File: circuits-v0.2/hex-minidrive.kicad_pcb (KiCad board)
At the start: 2 copper layers, 30 x 30 mm, 14 parts

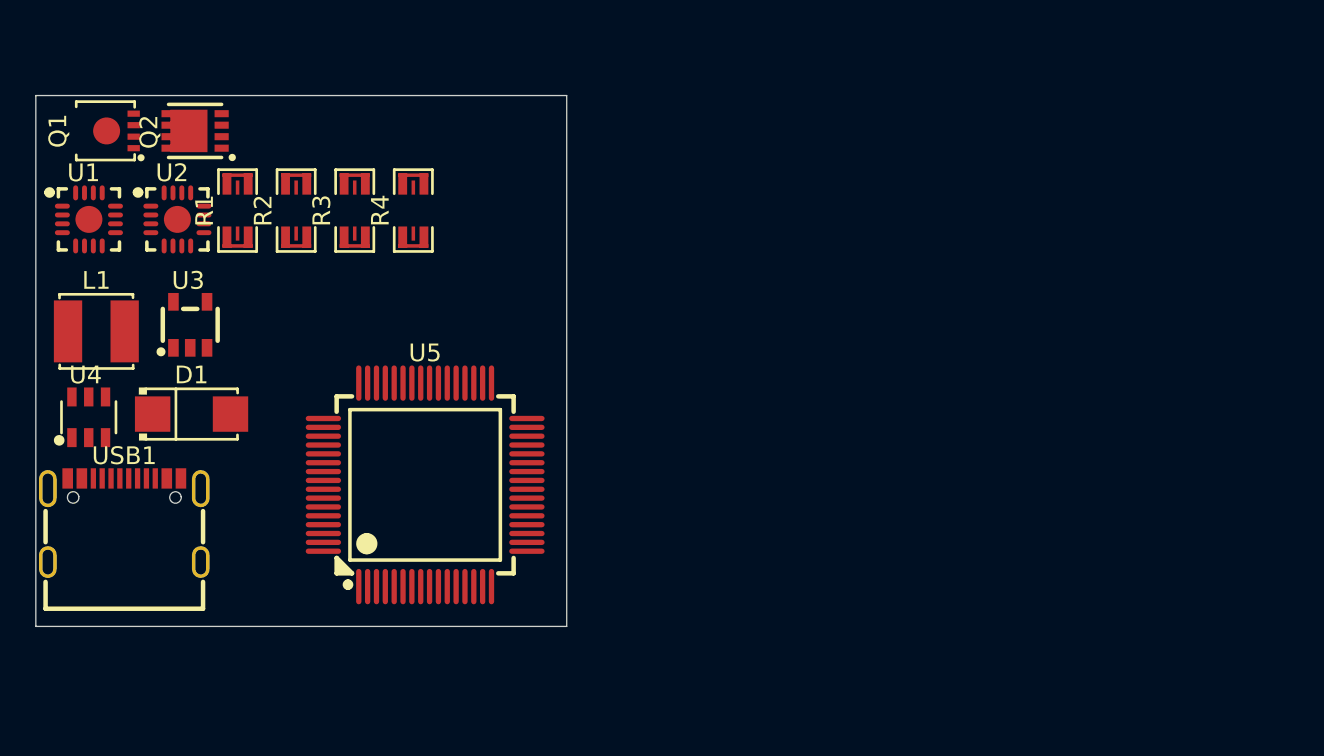
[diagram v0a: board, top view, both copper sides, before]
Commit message: Tentatively finish new schematic.
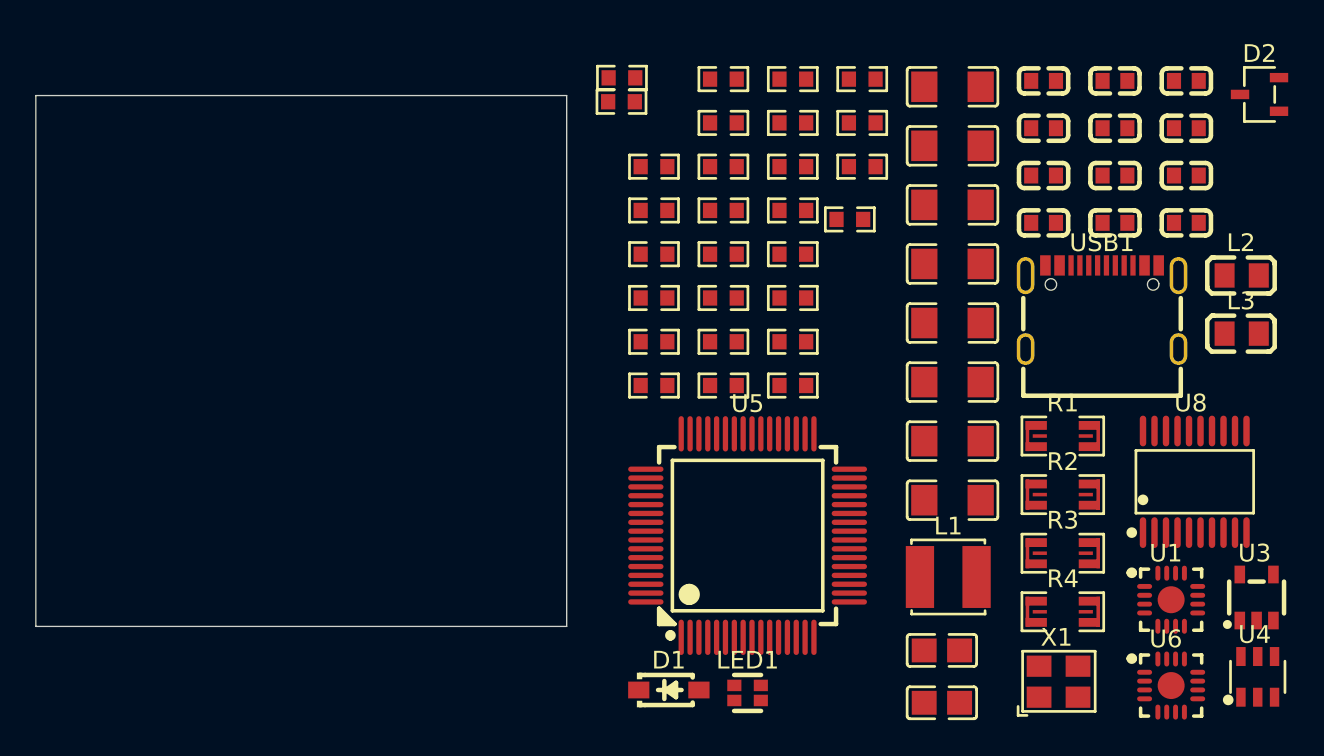
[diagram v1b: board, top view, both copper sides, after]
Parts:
- removed Q1: ~, Library:DFN-8_L3.3-W3.3-P0.65-BL-2
- removed Q2: ~, Library:DFN-8_L3.0-W3.0-P0.65-BL
- removed U2: ~, Library:QFN-16_L3.0-W3.0-P0.50-TL-EP1.7
- added C10: 10uF, Library:C1206, F.Cu at (97.8, 43.8)
- added C11: 10uF, Library:C1206, F.Cu at (97.8, 47.2)
- added C12: 1uF, Library:C0603, F.Cu at (107.0, 40.2)
- added C14: 10uF, Library:C1206, F.Cu at (97.8, 50.5)
- added C15: 10uF, Library:C1206, F.Cu at (97.8, 53.9)
- added C16: 10uF, Library:C1206, F.Cu at (97.8, 57.2)
- added C17: 10uF, Library:C1206, F.Cu at (97.8, 60.5)
- added C20: 15pF, Library:C0603, F.Cu at (107.0, 42.8)
- added C21: 15pF, Library:C0603, F.Cu at (107.0, 45.5)
- added C23: 1uF, Library:C0603, F.Cu at (107.0, 48.2)
- added C28: 10uF, Library:C1206, F.Cu at (97.8, 63.9)
- added C3: 10uF, Library:C1206, F.Cu at (97.8, 40.5)
- added C30: 1nF, Library:C0603, F.Cu at (111.0, 40.2)
- added C31: 1nF, Library:C0603, F.Cu at (111.0, 42.8)
- added C32: 1nF, Library:C0603, F.Cu at (111.0, 45.5)
- added C33: 1nF, Library:C0603, F.Cu at (111.0, 48.2)
- added C4: 22uF, Library:C0805, F.Cu at (97.2, 72.4)
- added C5: 22uF, Library:C0805, F.Cu at (97.2, 75.3)
- added C6: 100pF, Library:C0603, F.Cu at (102.9, 40.2)
- added C7: 1uF, Library:C0603, F.Cu at (102.9, 42.8)
- added C8: 1uF, Library:C0603, F.Cu at (102.9, 45.5)
- added C9: 10nF, Library:C0603, F.Cu at (102.9, 48.2)
- added D2: ~, Library:SOT-23-3_L3.0-W1.7-P0.95-LS2.9-BR, F.Cu at (115.2, 40.9)
- added L2: 10uH, Library:L0805, F.Cu at (114.1, 51.2)
- added L3: 300mΩ, Library:L0805, F.Cu at (114.1, 54.5)
- added LED1: ~, Library:LED-ARRAY-SMD_4P-L1.6-W1.5-BR_XL-1615RGBC-RF, F.Cu at (86.2, 74.8)
- added R10: 49.9Ω, Library:R0603, F.Cu at (80.9, 52.4)
- added R11: 1.5kΩ, Library:R0603, F.Cu at (80.9, 54.9)
- added R12: 1.5kΩ, Library:R0603, F.Cu at (80.9, 57.4)
- added R13: 1.5kΩ, Library:R0603, F.Cu at (84.9, 40.1)
- added R14: 10Ω, Library:R0603, F.Cu at (84.9, 42.5)
- added R15: 10Ω, Library:R0603, F.Cu at (84.9, 45.0)
- added R16: 10kΩ, Library:R0603, F.Cu at (84.9, 47.5)
- added R17: 100kΩ, Library:R0603, F.Cu at (84.9, 50.0)
- added R18: 10kΩ, Library:R0603, F.Cu at (84.9, 52.4)
- added R19: 10kΩ, Library:R0603, F.Cu at (84.9, 54.9)
- added R20: 10Ω, Library:R0603, F.Cu at (84.9, 57.4)
- added R21: 100kΩ, Library:R0603, F.Cu at (88.8, 40.1)
- added R22: 10Ω, Library:R0603, F.Cu at (88.8, 42.5)
- added R23: 10Ω, Library:R0603, F.Cu at (88.8, 45.0)
- added R24: 10Ω, Library:R0603, F.Cu at (88.8, 47.5)
- added R25: 5.1kΩ, Library:R0603, F.Cu at (88.8, 50.0)
- added R26: 10Ω, Library:R0603, F.Cu at (88.8, 52.4)
- added R27: 10Ω, Library:R0603, F.Cu at (88.8, 54.9)
- added R28: 100kΩ, Library:R0603, F.Cu at (88.8, 57.4)
- added R29: 10Ω, Library:R0603, F.Cu at (92.7, 40.1)
- added R30: 5.1kΩ, Library:R0603, F.Cu at (92.7, 42.5)
- added R31: 100kΩ, Library:R0603, F.Cu at (92.7, 45.0)
- added R33: 5.1kΩ, Library:R0603, F.Cu at (92.0, 48.0)
- added R5: 100kΩ, Library:R0603, F.Cu at (79.1, 40.0)
- added R6: 13kΩ, Library:R0603, F.Cu at (79.1, 41.4)
- added R7: 5.1kΩ, Library:R0603, F.Cu at (80.9, 45.0)
- added R8: 5.1kΩ, Library:R0603, F.Cu at (80.9, 47.5)
- added R9: 10Ω, Library:R0603, F.Cu at (80.9, 50.0)
- added U6: ~, Library:QFN-16_L3.0-W3.0-P0.50-TL-EP1.7, F.Cu at (110.2, 74.3)
- added U8: ~, Library:TSSOP-20_L6.5-W4.4-P0.65-LS6.4-BL, F.Cu at (111.5, 62.8)
- added X1: 16MHz, Library:OSC-SMD_4P-L3.2-W2.5-BL, F.Cu at (103.8, 74.1)
- D1: footprint Library:SMA_L4.3-W2.6-LS5.2-RD -> Library:SOD-123_L2.7-W1.6-LS3.7-RD-1
- moved U4 67.7 mm to (115.0, 73.9)
- moved U1 64.8 mm to (110.2, 69.5)
- moved U3 62.2 mm to (115.0, 69.4)
- moved USB1 56.5 mm to (106.3, 53.0)
- moved L1 50.1 mm to (97.6, 68.2)
- moved R1 48.3 mm to (104.0, 60.2), turned to 0 degrees
- moved R2 46.2 mm to (104.0, 63.6), turned to 0 degrees
- moved R3 44.5 mm to (104.0, 66.9), turned to 0 degrees
- moved R4 43.1 mm to (104.0, 70.2), turned to 0 degrees
- moved D1 31.2 mm to (81.8, 74.6)
- moved U5 18.4 mm to (86.2, 65.9)
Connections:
- D1 pad 1: unconnected-(D1-K-Pad1) -> 5V
- D1 pad 2: unconnected-(D1-A-Pad2) -> Net-(D1-+)
- L1 pad 1: unconnected-(L1-Pad1) -> Net-(U4-SW)
- L1 pad 2: unconnected-(L1-Pad2) -> 5V
- R1 pad 1: unconnected-(R1-Shunt-1-Pad1) -> Net-(Q1-S)
- R1 pad 2: unconnected-(R1-Shunt-2-Pad2) -> GND
- R1 pad 3: unconnected-(R1-Probe-1-Pad3) -> +Probe-1
- R1 pad 4: unconnected-(R1-Probe-2-Pad4) -> -Probe-1
- R2 pad 1: unconnected-(R2-Shunt-1-Pad1) -> Net-(Q3-S)
- R2 pad 2: unconnected-(R2-Shunt-2-Pad2) -> GND
- R2 pad 3: unconnected-(R2-Probe-1-Pad3) -> +Probe-2
- R2 pad 4: unconnected-(R2-Probe-2-Pad4) -> -Probe-2
- R3 pad 1: unconnected-(R3-Shunt-1-Pad1) -> Net-(Q5-S)
- R3 pad 2: unconnected-(R3-Shunt-2-Pad2) -> GND
- R3 pad 3: unconnected-(R3-Probe-1-Pad3) -> +Probe-3
- R3 pad 4: unconnected-(R3-Probe-2-Pad4) -> -Probe-3
- R4 pad 1: unconnected-(R4-Shunt-1-Pad1) -> Net-(Q7-S)
- R4 pad 2: unconnected-(R4-Shunt-2-Pad2) -> GND
- R4 pad 3: unconnected-(R4-Probe-1-Pad3) -> +Probe-4
- R4 pad 4: unconnected-(R4-Probe-2-Pad4) -> -Probe-4
- U1 pad 1: unconnected-(U1-HIN1-Pad1) -> TIM1_CH1
- U1 pad 10: unconnected-(U1-HO2-Pad10) -> P-Gate-2
- U1 pad 11: unconnected-(U1-LO2-Pad11) -> N-Gate-2
- U1 pad 14: unconnected-(U1-GND-Pad14) -> GND
- U1 pad 16: unconnected-(U1-HIN2-Pad16) -> TIM1_CH2
- U1 pad 3: unconnected-(U1-LIN2-Pad3) -> TIM1_CH2N
- U1 pad 4: unconnected-(U1-LIN1-Pad4) -> TIM1_CH1N
- U1 pad 6: unconnected-(U1-VCC1-Pad6) -> Net-(U1-VCC1)
- U1 pad 7: unconnected-(U1-VCC2-Pad7) -> VCC
- U1 pad 8: unconnected-(U1-HO1-Pad8) -> P-Gate-1
- U1 pad 9: unconnected-(U1-LO1-Pad9) -> N-Gate-1
- U3 pad 1: unconnected-(U3-IN-Pad1) -> 5V
- U3 pad 2: unconnected-(U3-GND-Pad2) -> GND
- U3 pad 3: unconnected-(U3-EN-Pad3) -> 5V
- U3 pad 4: unconnected-(U3-BYP-Pad4) -> Net-(U3-BYP)
- U3 pad 5: unconnected-(U3-OUT-Pad5) -> 3V3
- U4 pad 1: unconnected-(U4-GND-Pad1) -> GND
- U4 pad 2: unconnected-(U4-SW-Pad2) -> Net-(U4-SW)
- U4 pad 3: unconnected-(U4-VIN-Pad3) -> VCC
- U4 pad 4: unconnected-(U4-FB-Pad4) -> Buck-FB
- U4 pad 6: unconnected-(U4-BOOT-Pad6) -> Net-(U4-BOOT)
- U5 pad 16: unconnected-(U5-VDD-Pad16) -> 3V3
- U5 pad 32: unconnected-(U5-VDD-Pad32) -> 3V3
- U5 pad 48: unconnected-(U5-VDD-Pad48) -> 3V3
- U5 pad 5: unconnected-(U5-PF0-OSC_IN-Pad5) -> Net-(U5-PF0-OSC_IN)
- U5 pad 6: unconnected-(U5-PF1-OSC_OUT-Pad6) -> Net-(U5-PF1-OSC_OUT)
- U5 pad 64: unconnected-(U5-VDD-Pad64) -> 3V3
- USB1 pad A1B12: unconnected-(USB1-GND-PadA1B12) -> GND
- USB1 pad A4B9: unconnected-(USB1-VBUS-PadA4B9) -> USB:5V
- USB1 pad A5: unconnected-(USB1-CC1-PadA5) -> Net-(USB1-CC1)
- USB1 pad A6: unconnected-(USB1-DP1-PadA6) -> USB_D_P
- USB1 pad A7: unconnected-(USB1-DN1-PadA7) -> USB_D_N
- USB1 pad B1A12: unconnected-(USB1-GND-PadB1A12) -> GND
- USB1 pad B4A9: unconnected-(USB1-VBUS-PadB4A9) -> USB:5V
- USB1 pad B5: unconnected-(USB1-CC2-PadB5) -> Net-(USB1-CC2)
- USB1 pad B6: unconnected-(USB1-DP2-PadB6) -> USB_D_P
- USB1 pad B7: unconnected-(USB1-DN2-PadB7) -> USB_D_N

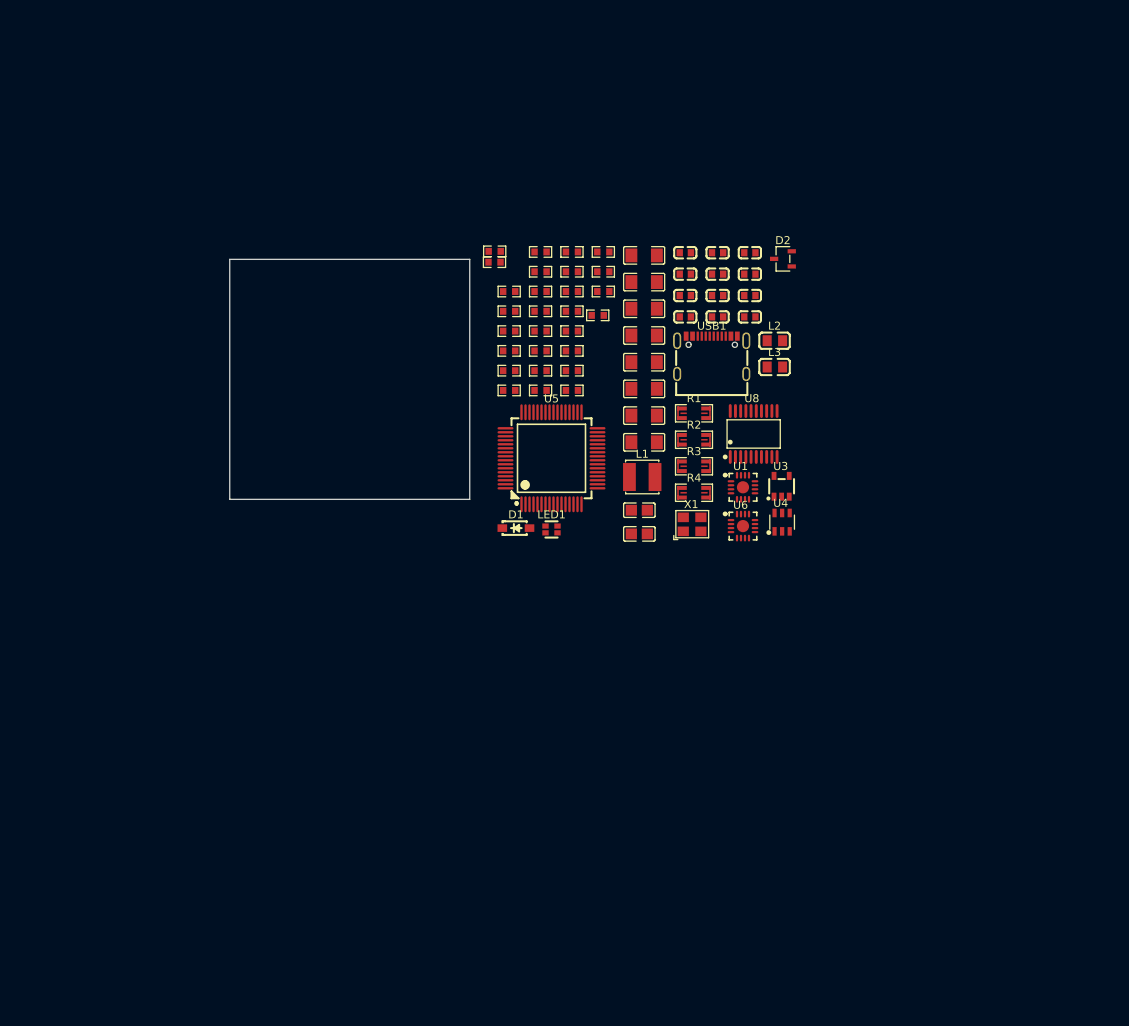
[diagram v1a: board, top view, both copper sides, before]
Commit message: Finish the new version schematic.
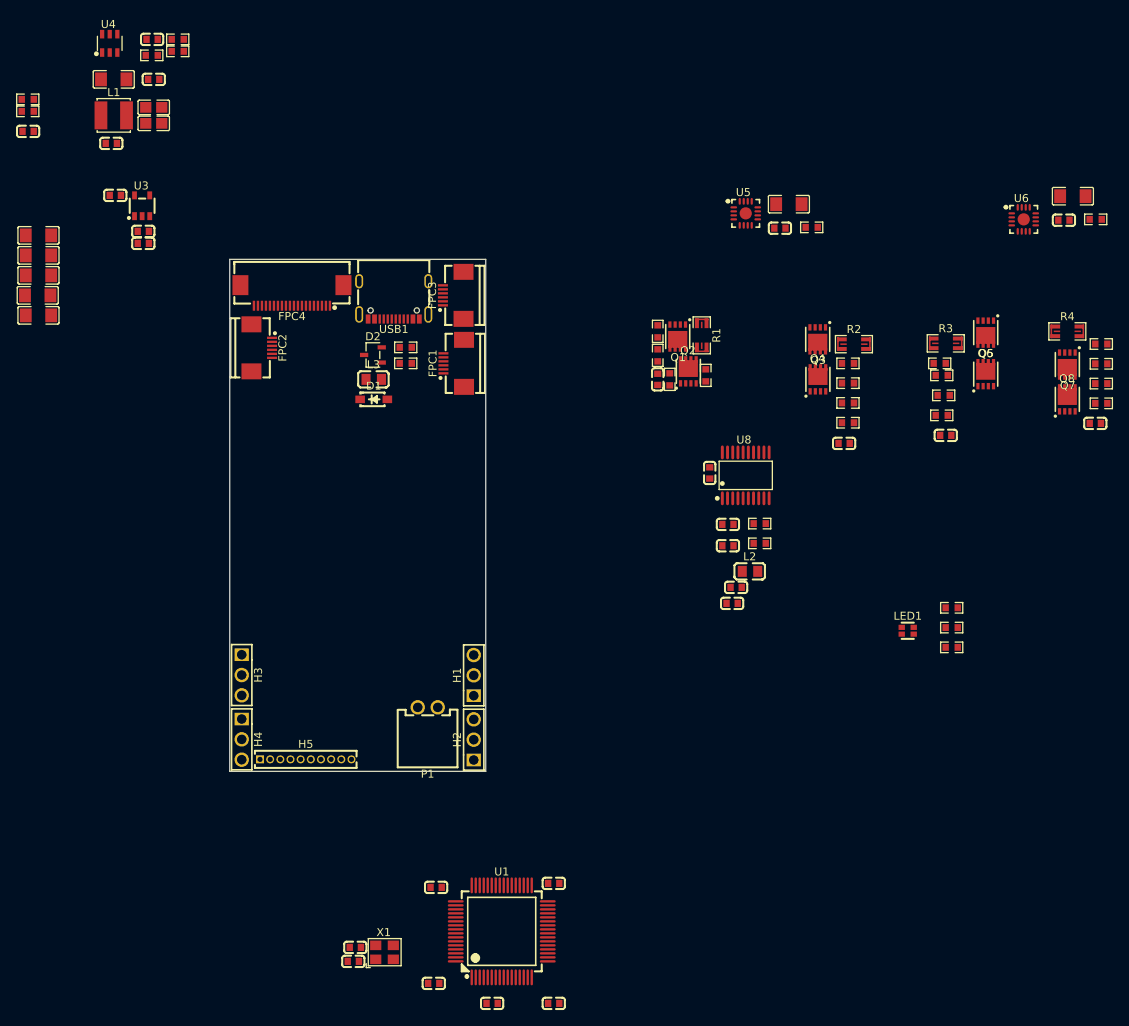
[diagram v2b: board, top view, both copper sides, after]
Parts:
- removed C17, C28: 10uF, Library:C1206
- removed C23: 1uF, Library:C0603
- removed C31, C32, C33: 1nF, Library:C0603
- removed R13: 1.5kΩ, Library:R0603
- removed R14, R15, R20, R24, R26, R27, R29, R9: 10Ω, Library:R0603
- removed R16, R19: 10kΩ, Library:R0603
- removed R25, R30, R33, R7, R8: 5.1kΩ, Library:R0603
- removed R28, R31: 100kΩ, Library:R0603
- added C1: 100nF, Library:C0603, F.Cu at (31.2, 26.5)
- added C101: 1nF, Library:C0603, F.Cu at (99.5, 56.0)
- added C13: 100nF, Library:C0603, F.Cu at (108.8, 84.0)
- added C2: 100nF, Library:C0603, F.Cu at (36.5, 18.5)
- added C201: 1nF, Library:C0603, F.Cu at (122.8, 64.0)
- added C24: 100nF, Library:C0603, F.Cu at (86.5, 134.0)
- added C25: 100nF, Library:C0603, F.Cu at (86.5, 119.0)
- added C26: 100nF, Library:C0603, F.Cu at (71.8, 119.5)
- added C27: 100nF, Library:C0603, F.Cu at (71.5, 131.5)
- added C301: 1nF, Library:C0603, F.Cu at (135.5, 63.0)
- added C34: 10nF, Library:C0603, F.Cu at (78.8, 134.0)
- added C401: 1nF, Library:C0603, F.Cu at (154.2, 61.5)
- added C501: 10uF, Library:C1206, F.Cu at (115.9, 34.1)
- added C502: 100nF, Library:C0603, F.Cu at (114.8, 37.1)
- added C601: 10uF, Library:C1206, F.Cu at (151.4, 33.1)
- added C602: 100nF, Library:C0603, F.Cu at (150.3, 36.1)
- added C801: 100nF, Library:C0603, F.Cu at (106.0, 67.7)
- added C802: 100nF, Library:C0603, F.Cu at (108.3, 74.1)
- added C803: 1uF, Library:C0603, F.Cu at (108.3, 76.8)
- added FPC1: ~, Library:FPC-SMD_6P-P0.50_XUNPU_FPC-05F-6PH20, F.Cu at (74.0, 54.0)
- added FPC2: ~, Library:FPC-SMD_6P-P0.50_XUNPU_FPC-05F-6PH20, F.Cu at (50.0, 52.1)
- added FPC3: ~, Library:FPC-SMD_6P-P0.50_XUNPU_FPC-05F-6PH20, F.Cu at (73.9, 45.5)
- added FPC4: ~, Library:FPC-SMD_20P-P0.50_XUNPU_FPC-05F-20PH20, F.Cu at (53.8, 45.5)
- added H1: 2.54mm 3P header, Library:HDR-TH_3P-P2.54-V-M-1, F.Cu at (76.5, 93.0)
- added H2: 2.54mm 3P header, Library:HDR-TH_3P-P2.54-V-M-1, F.Cu at (76.5, 101.0)
- added H3: 2.54mm 3P header, Library:HDR-TH_3P-P2.54-V-M-1, F.Cu at (47.5, 93.0)
- added H4: 2.54mm 3P header, Library:HDR-TH_3P-P2.54-V-M-1, F.Cu at (47.5, 101.0)
- added H5: 10P 1.27mm header, Library:HDR-TH_HX-PZ1.27-1X10P-ZZ, F.Cu at (55.5, 103.5)
- added P1: 2P 2.54mm header, Library:CONN-TH_2P-P2.50_XH-2AW, F.Cu at (70.8, 97.0)
- added Q1: ~, Library:DFN-8_L3.0-W3.0-P0.65-BL-MOSFET, F.Cu at (102.0, 50.6)
- added Q2: ~, Library:DFN-8_L3.0-W3.0-P0.65-BL-MOSFET, F.Cu at (103.3, 55.0)
- added Q3: ~, Library:DFN-8_L3.0-W3.0-P0.65-BL-MOSFET, F.Cu at (119.5, 51.0)
- added Q4: ~, Library:DFN-8_L3.0-W3.0-P0.65-BL-MOSFET, F.Cu at (119.5, 56.0)
- added Q5: ~, Library:DFN-8_L3.0-W3.0-P0.65-BL-MOSFET, F.Cu at (140.5, 50.2)
- added Q6: ~, Library:DFN-8_L3.0-W3.0-P0.65-BL-MOSFET, F.Cu at (140.5, 55.4)
- added Q7: ~, Library:DFN-8_L3.0-W3.0-P0.65-BL-MOSFET, F.Cu at (150.7, 54.1)
- added Q8: ~, Library:DFN-8_L3.0-W3.0-P0.65-BL-MOSFET, F.Cu at (150.7, 58.5)
- added R101: 10Ω, Library:R0603, F.Cu at (99.5, 50.0)
- added R102: 10Ω, Library:R0603, F.Cu at (105.5, 55.5)
- added R103: 100kΩ, Library:R0603, F.Cu at (99.5, 53.0)
- added R104: 5.1kΩ, Library:R0603, F.Cu at (101.0, 56.0)
- added R201: 10Ω, Library:R0603, F.Cu at (123.3, 54.0)
- added R202: 10Ω, Library:R0603, F.Cu at (123.3, 56.5)
- added R203: 100kΩ, Library:R0603, F.Cu at (123.3, 58.9)
- added R204: 5.1kΩ, Library:R0603, F.Cu at (123.3, 61.4)
- added R301: 10Ω, Library:R0603, F.Cu at (134.7, 54.0)
- added R302: 10Ω, Library:R0603, F.Cu at (135.0, 55.5)
- added R303: 100kΩ, Library:R0603, F.Cu at (135.2, 58.0)
- added R304: 5.1kΩ, Library:R0603, F.Cu at (135.0, 60.5)
- added R401: 10Ω, Library:R0603, F.Cu at (154.9, 51.6)
- added R402: 10Ω, Library:R0603, F.Cu at (154.9, 54.1)
- added R403: 100kΩ, Library:R0603, F.Cu at (154.9, 56.5)
- added R404: 5.1kΩ, Library:R0603, F.Cu at (154.9, 59.0)
- added R501: 10Ω, Library:R0603, F.Cu at (118.7, 37.0)
- added R601: 10Ω, Library:R0603, F.Cu at (154.2, 36.0)
- added R801: 10kΩ, Library:R0603, F.Cu at (112.2, 74.0)
- added R802: 10kΩ, Library:R0603, F.Cu at (112.2, 76.5)
- R11, R12: value 1.5kΩ -> 5.1kΩ
- R21: value 100kΩ -> 1.5kΩ
- R22, R23: value 10Ω -> 1.5kΩ
- U1: footprint Library:QFN-16_L3.0-W3.0-P0.50-TL-EP1.7 -> Library:LQFP-64_L10.0-W10.0-P0.50-LS12.0-BL
- U5: footprint Library:LQFP-64_L10.0-W10.0-P0.50-LS12.0-BL -> Library:QFN-16_L3.0-W3.0-P0.50-TL-EP1.7
- moved U4 103.2 mm to (31.0, 14.0)
- moved C20 97.2 mm to (61.5, 128.8)
- moved C21 93.2 mm to (61.7, 127.0)
- moved C30 91.5 mm to (20.8, 25.0)
- moved U3 87.3 mm to (35.0, 34.3)
- moved L1 80.0 mm to (31.5, 23.0)
- moved C5 79.5 mm to (36.5, 24.0)
- moved C4 78.9 mm to (36.5, 22.0), turned to 180 degrees
- moved C16 76.3 mm to (22.1, 48.0)
- moved C15 76.3 mm to (22.0, 45.5)
- moved C14 76.1 mm to (22.1, 43.0)
- moved C11 76.0 mm to (22.1, 40.5)
- moved C10 75.9 mm to (22.1, 38.0)
- moved C7 71.9 mm to (31.7, 33.0)
- moved C6 71.8 mm to (36.3, 13.5)
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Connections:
- C20 pad 2: Net-(U5-PF0-OSC_IN) -> Net-(U1-PF0-OSC_IN)
- C21 pad 2: Net-(U5-PF1-OSC_OUT) -> Net-(U1-PF1-OSC_OUT)
- C30 pad 2: ADC1_IN? -> ADC2_IN15/VOLTAGE
- R11 pad 1: unconnected-(R11-Pad1) -> GND
- R11 pad 2: Net-(LED1-R-) -> Net-(USB1-CC1)
- R12 pad 1: Net-(LED1-G-) -> GND
- R12 pad 2: unconnected-(R12-Pad2) -> Net-(USB1-CC2)
- R17 pad 1: ADC1_IN? -> ADC2_IN15/VOLTAGE
- R18 pad 2: ADC1_IN? -> ADC2_IN15/VOLTAGE
- R21 pad 1: ADC1_IN? -> TIM4_CH1/RED_LED
- R21 pad 2: M1 -> Net-(LED1-R-)
- R22 pad 1: Net-(Q4-G) -> Net-(LED1-G-)
- R22 pad 2: P-Gate-2 -> TIM4_CH2/GREEN_LED
- R23 pad 1: N-Gate-3 -> Net-(LED1-B-)
- R23 pad 2: Net-(Q5-G) -> TIM2_CH3/BLUE_LED
- U1 pad 1: TIM1_CH1 -> 3V3
- U1 pad 10: P-Gate-2 -> ADC1_IN8/POT_2
- U1 pad 11: N-Gate-2 -> TIM1_CH4
- U1 pad 12: unconnected-(U1-HO3-Pad12) -> ADC1_IN1/M1_CURRENT
- U1 pad 13: unconnected-(U1-LO3-Pad13) -> OPAMP1_VINP/M1_VOLTAGE
- U1 pad 14: GND -> ADC1_IN3/HALF_3V3_REF
- U1 pad 15: unconnected-(U1-HIN3-Pad15) -> GND
- U1 pad 16: TIM1_CH2 -> 3V3
- U1 pad 17: unconnected-(U1-EP-Pad17) -> ADC1_IN3/HALF_3V3_REF
- U1 pad 2: unconnected-(U1-LIN3-Pad2) -> TIM1_CH1N
- U1 pad 3: TIM1_CH2N -> FREE_IO_1
- U1 pad 4: TIM1_CH1N -> FREE_IO_2
- U1 pad 5: unconnected-(U1-5V-Pad5) -> Net-(U1-PF0-OSC_IN)
- U1 pad 6: Net-(U1-VCC1) -> Net-(U1-PF1-OSC_OUT)
- U1 pad 7: VCC -> NRST
- U1 pad 8: P-Gate-1 -> TIM1_CH1
- U1 pad 9: N-Gate-1 -> ADC1_IN7/POT_1
- U5 pad 1: unconnected-(U5-VBAT-Pad1) -> TIM1_CH1
- U5 pad 10: unconnected-(U5-PC2-Pad10) -> P-Gate-2
- U5 pad 11: unconnected-(U5-PC3-Pad11) -> N-Gate-2
- U5 pad 14: unconnected-(U5-PA2-Pad14) -> GND
- U5 pad 15: unconnected-(U5-VSS-Pad15) -> GND
- U5 pad 16: 3V3 -> TIM1_CH2
- U5 pad 2: unconnected-(U5-PC13-Pad2) -> GND
- U5 pad 3: unconnected-(U5-PC14-OSC32_IN-Pad3) -> TIM1_CH2N
- U5 pad 4: unconnected-(U5-PC15-OSC32_OUT-Pad4) -> TIM1_CH1N
- U5 pad 5: Net-(U5-PF0-OSC_IN) -> unconnected-(U5-5V-Pad5)
- U5 pad 6: Net-(U5-PF1-OSC_OUT) -> Net-(U5-VCC1)
- U5 pad 7: unconnected-(U5-PG10-NRST-Pad7) -> VCC
- U5 pad 8: unconnected-(U5-PC0-Pad8) -> P-Gate-1
- U5 pad 9: unconnected-(U5-PC1-Pad9) -> N-Gate-1
- U6 pad 15: unconnected-(U6-HIN3-Pad15) -> GND
- U6 pad 2: unconnected-(U6-LIN3-Pad2) -> GND
- U8 pad 1: ADC1_IN5/REF -> ADC1_IN3/HALF_3V3_REF
- U8 pad 12: ADC1_IN5/REF -> ADC1_IN3/HALF_3V3_REF
- U8 pad 13: unconnected-(U8-OUT3-Pad13) -> ADC1_IN12/M3_CURRENT
- U8 pad 19: unconnected-(U8-OUT4-Pad19) -> ADC2_IN14/M4_CURRENT
- U8 pad 2: unconnected-(U8-OUT1-Pad2) -> ADC1_IN1/M1_CURRENT
- U8 pad 20: ADC1_IN5/REF -> ADC1_IN3/HALF_3V3_REF
- U8 pad 8: unconnected-(U8-OUT2-Pad8) -> ADC2_IN3/M2_CURRENT
- U8 pad 9: ADC1_IN5/REF -> ADC1_IN3/HALF_3V3_REF
- X1 pad 1: Net-(U5-PF0-OSC_IN) -> Net-(U1-PF0-OSC_IN)
- X1 pad 3: Net-(U5-PF1-OSC_OUT) -> Net-(U1-PF1-OSC_OUT)
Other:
- board size 30 x 30 mm -> 32 x 64 mm
